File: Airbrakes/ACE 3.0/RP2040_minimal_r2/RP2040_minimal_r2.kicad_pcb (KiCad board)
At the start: 2 copper layers, 52 x 51 mm, 44 parts, among them J1 USB_B_Micro, J2 Conn_01x02, J3 104031-0811, J4 Conn_02x18_Odd_Even, U1 NCP1117-3.3_SOT223, U2 W25Q128JVS, U3 RP2040, U4 BMI088, U5 BMP581, U6 BMM350, Y1 ABM8-272-T3

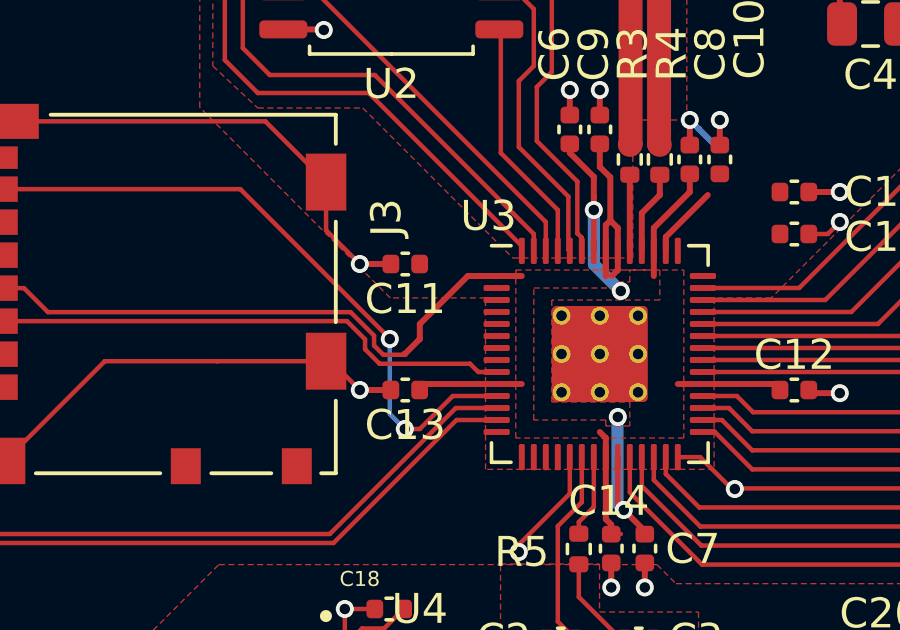
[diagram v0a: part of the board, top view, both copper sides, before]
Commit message: Update traces
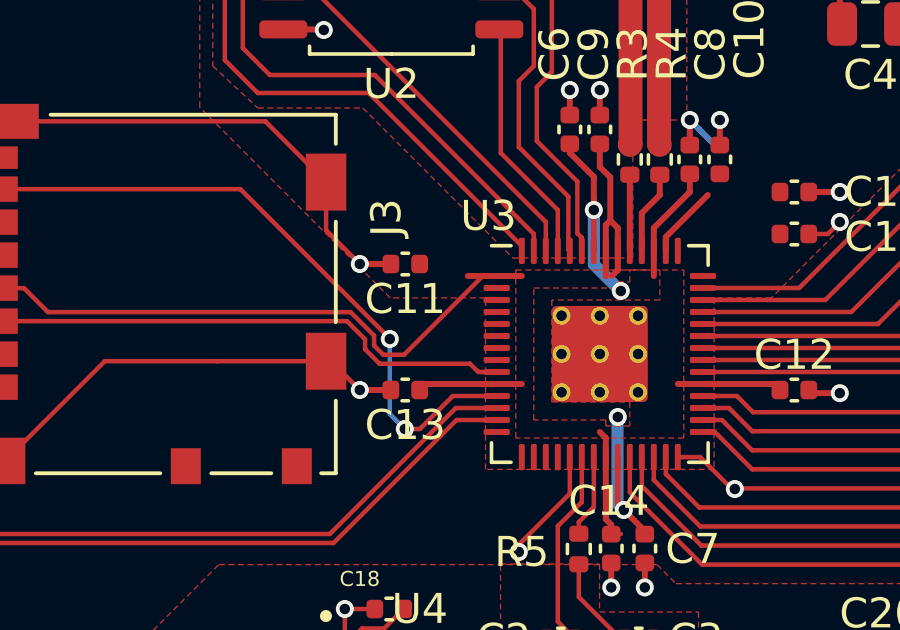
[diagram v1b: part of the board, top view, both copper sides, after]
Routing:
- net +3V3: track 61.6 -> 62.3 mm
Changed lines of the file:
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@@
+	)
+	(segment
+		(start 92.475 99.717463)
+		(end 92.782537 100.025)
+		(width 0.15)
+		(layer "F.Cu")
+		(net 5)
 	)
 	(segment
@@
 	)
 	(segment
-		(start 95.6 97.4)
-		(end 94 99)
-		(width 0.2)
-		(layer "F.Cu")
-		(net 5)
-	)
-	(segment
 		(start 100.2 95.7)
 		(end 100.2 96.5625)
@@
 	)
 	(segment
+		(start 92.782537 100.025)
+		(end 93.475 100.025)
+		(width 0.15)
+		(layer "F.Cu")
+		(net 5)
+	)
+	(segment
 		(start 100.350001 94.112535)
 		(end 100.350001 95.549999)
@@
 	)
 	(segment
-		(start 93.5 100)
-		(end 93.475 100)
-		(width 0.2)
-		(layer "F.Cu")
-		(net 5)
-	)
-	(segment
 		(start 93 112.5)
 		(end 93 112)
@@
 	)
 	(segment
+		(start 96.1 97.4)
+		(end 96.5625 97.4)
+		(width 0.15)
+		(layer "F.Cu")
+		(net 5)
+	)
+	(segment
 		(start 100.6 96.5625)
 		(end 100.6 97.2)
@@
 	)
 	(segment
-		(start 92.782537 100.025)
-		(end 93.475 100.025)
-		(width 0.15)
-		(layer "F.Cu")
-		(net 5)
-	)
-	(segment
 		(start 88.905 81.805)
 		(end 89.5 81.805)
@@
 	)
 	(segment
+		(start 80.805 97.805)
+		(end 81.605 98.605)
+		(width 0.15)
+		(layer "F.Cu")
+		(net 5)
+	)
+	(segment
+		(start 80.05 97.805)
+		(end 80.805 97.805)
+		(width 0.15)
+		(layer "F.Cu")
+		(net 5)
+	)
+	(segment
 		(start 100.6 96.5625)
 		(end 100.6 95.799998)
@@
 	)
 	(segment
-		(start 94 99)
-		(end 94 99.5)
+		(start 100.2 96.5625)
+		(end 100.2 97.4)
+		(width 0.2)
+		(layer "F.Cu")
+		(net 5)
+	)
+	(segment
+		(start 108 86)
+		(end 108 89)
+		(width 0.2)
+		(layer "F.Cu")
+		(net 5)
+	)
+	(segment
+		(start 100.381 105.6865)
+		(end 100.381 106)
+		(width 0.2)
+		(layer "F.Cu")
+		(net 5)
+	)
+	(segment
+		(start 100.350001 95.549999)
+		(end 100.2 95.7)
+		(width 0.2)
+		(layer "F.Cu")
+		(net 5)
+	)
+	(segment
+		(start 80.05 97.805)
+		(end 79.805 97.805)
+		(width 0.15)
+		(layer "F.Cu")
+		(net 5)
+	)
+	(segment
+		(start 102.2 96.1)
+		(end 103.6 94.7)
+		(width 0.2)
+		(layer "F.Cu")
+		(net 5)
+	)
+	(segment
+		(start 92.81 109.15)
+		(end 93.46 108.5)
+		(width 0.15)
+		(layer "F.Cu")
+		(net 5)
+	)
+	(segment
+		(start 100.2 97.4)
+		(end 100.2 97)
+		(width 0.2)
+		(layer "F.Cu")
+		(net 5)
+	)
+	(segment
+		(start 81.605 98.605)
+		(end 91.694332 98.605)
+		(width 0.15)
+		(layer "F.Cu")
+		(net 5)
+	)
+	(segment
+		(start 100 93.762534)
+		(end 100.350001 94.112535)
+		(width 0.2)
+		(layer "F.Cu")
+		(net 5)
+	)
+	(segment
+		(start 93.475 100.025)
+		(end 96.1 97.4)
+		(width 0.15)
+		(layer "F.Cu")
+		(net 5)
+	)
+	(segment
+		(start 92 109.67)
+		(end 92 109.225)
+		(width 0.15)
+		(layer "F.Cu")
+		(net 5)
+	)
+	(segment
+		(start 96.65 85.37)
+		(end 96.65 82.85)
+		(width 0.2)
+		(layer "F.Cu")
+		(net 5)
+	)
+	(segment
+		(start 100.2 103.4375)
+		(end 100.2 102.8)
+		(width 0.2)
+		(layer "F.Cu")
+		(net 5)
+	)
+	(segment
+		(start 102.2 96.5625)
+		(end 102.2 96.1)
+		(width 0.2)
+		(layer "F.Cu")
+		(net 5)
+	)
+	(segment
+		(start 96.65 82.85)
+		(end 96.67 82.83)
 		(width 0.2)
 		(layer "F.Cu")
@@
 		(layer "F.Cu")
 		(net 5)
-	)
-	(segment
-		(start 100.2 96.5625)
-		(end 100.2 97.4)
-		(width 0.2)
-		(layer "F.Cu")
-		(net 5)
-	)
-	(segment
-		(start 108 86)
-		(end 108 89)
-		(width 0.2)
-		(layer "F.Cu")
-		(net 5)
-	)
-	(segment
-		(start 100.381 105.6865)
-		(end 100.381 106)
-		(width 0.2)
-		(layer "F.Cu")
-		(net 5)
-	)
-	(segment
-		(start 94 99.5)
-		(end 93.5 100)
-		(width 0.2)
-		(layer "F.Cu")
-		(net 5)
-	)
-	(segment
-		(start 92.475 99.717463)
-		(end 92.782537 100.025)
-		(width 0.15)
-		(layer "F.Cu")
-		(net 5)
-	)
-	(segment
-		(start 100.350001 95.549999)
-		(end 100.2 95.7)
-		(width 0.2)
-		(layer "F.Cu")
-		(net 5)
-	)
-	(segment
-		(start 80.05 97.805)
-		(end 79.805 97.805)
-		(width 0.15)
-		(layer "F.Cu")
-		(net 5)
-	)
-	(segment
-		(start 102.2 96.1)
-		(end 103.6 94.7)
-		(width 0.2)
-		(layer "F.Cu")
-		(net 5)
-	)
-	(segment
-		(start 92.81 109.15)
-		(end 93.46 108.5)
-		(width 0.15)
-		(layer "F.Cu")
-		(net 5)
-	)
-	(segment
-		(start 81.605 98.605)
-		(end 91.694332 98.605)
-		(width 0.15)
-		(layer "F.Cu")
-		(net 5)
-	)
-	(segment
-		(start 80.805 97.805)
-		(end 81.605 98.605)
-		(width 0.15)
-		(layer "F.Cu")
-		(net 5)
-	)
-	(segment
-		(start 100.2 97.4)
-		(end 100.2 97)
-		(width 0.2)
-		(layer "F.Cu")
-		(net 5)
-	)
-	(segment
-		(start 100 93.762534)
-		(end 100.350001 94.112535)
-		(width 0.2)
-		(layer "F.Cu")
-		(net 5)
-	)
-	(segment
-		(start 80.05 97.805)
-		(end 80.805 97.805)
-		(width 0.15)
-		(layer "F.Cu")
-		(net 5)
-	)
-	(segment
-		(start 92 109.67)
-		(end 92 109.225)
-		(width 0.15)
-		(layer "F.Cu")
-		(net 5)
-	)
-	(segment
-		(start 96.65 85.37)
-		(end 96.65 82.85)
-		(width 0.2)
-		(layer "F.Cu")
-		(net 5)
-	)
-	(segment
-		(start 100.2 103.4375)
-		(end 100.2 102.8)
-		(width 0.2)
-		(layer "F.Cu")
-		(net 5)
-	)
-	(segment
-		(start 102.2 96.5625)
-		(end 102.2 96.1)
-		(width 0.2)
-		(layer "F.Cu")
-		(net 5)
-	)
-	(segment
-		(start 96.65 82.85)
-		(end 96.67 82.83)
-		(width 0.2)
-		(layer "F.Cu")
-		(net 5)
